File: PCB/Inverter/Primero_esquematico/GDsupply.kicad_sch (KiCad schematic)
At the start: 43 parts, among them T1 750317595, U1 UCC21750QDWRQ1, U2 LM25180QNGURQ1

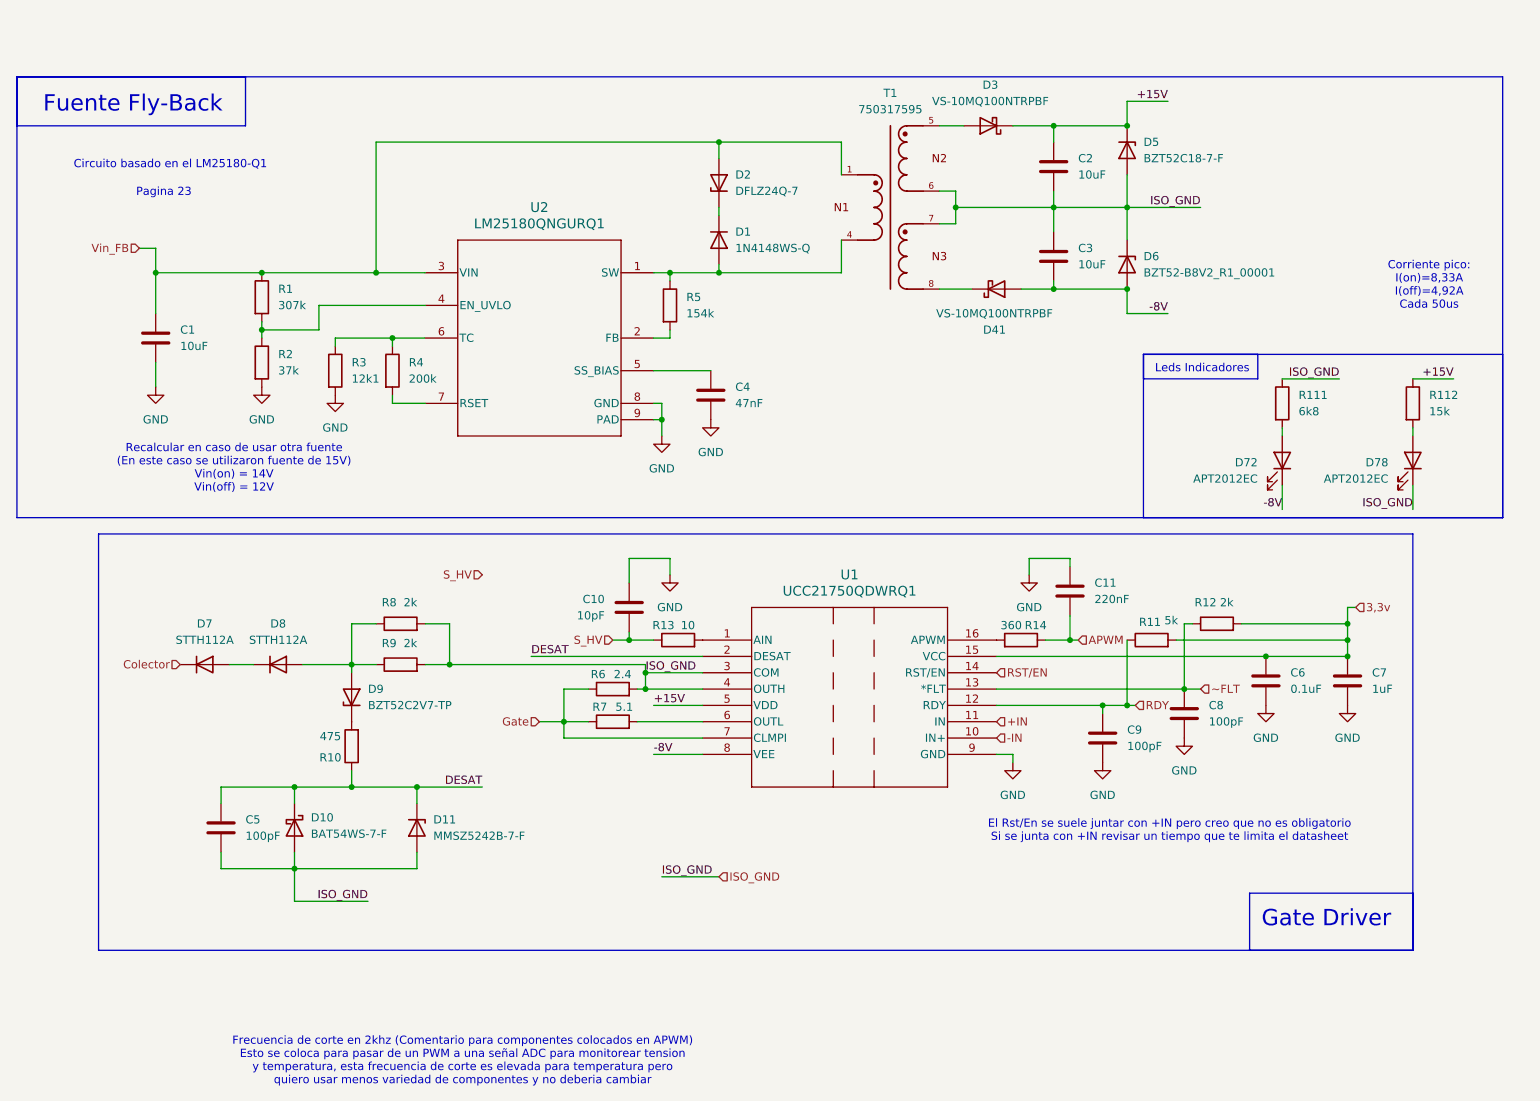
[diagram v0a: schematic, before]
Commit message: Correcciones incompletas e instalaciones de un par de extensiones copadas
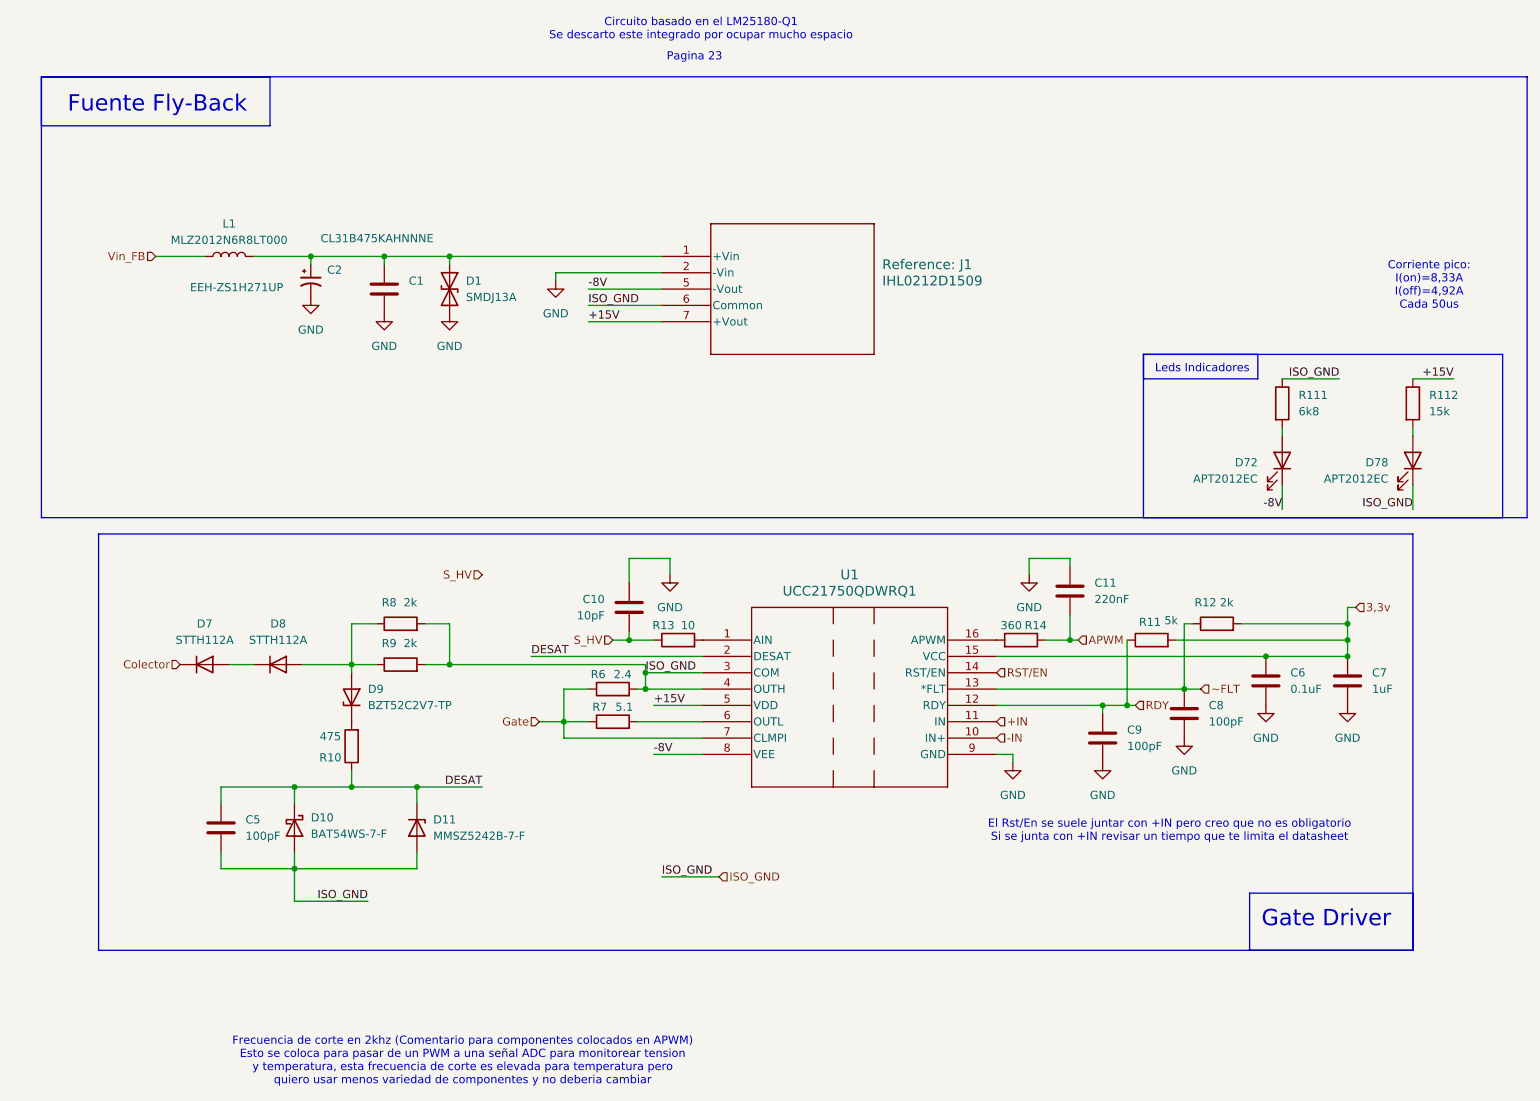
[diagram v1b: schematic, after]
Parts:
- removed C2, C3: 10uF, symbol Device:C
- removed C4: 47nF, symbol Device:C
- removed D1: 1N4148WS-Q, Diode_SMD:D_SOD-323F, symbol Device:D
- removed D2: DFLZ24Q-7, symbol Device:D_Zener
- removed D3, D41: VS-10MQ100NTRPBF, symbol Device:D_Schottky
- removed D5: BZT52C18-7-F, symbol Device:D_Zener
- removed D6: BZT52-B8V2_R1_00001, symbol Device:D_Zener
- removed R1: 307k, symbol Device:R
- removed R2: 37k, symbol Device:R
- removed R3: 12k1, symbol Device:R
- removed R4: 200k, symbol Device:R
- removed R5: 154k, symbol Device:R
- removed T1: 750317595, FSAE-footprints:WE-FLYTI_EP7_4436, symbol Fsae:750317595
- removed U2: LM25180QNGURQ1, NGU0008C, symbol Fsae:LM25180QNGURQ1
- added C2: EEH-ZS1H271UP, Capacitor_SMD:CP_Elec_10x10, symbol Device:C_Polarized_Small_US
- added D1: SMDJ13A, Diode_SMD:D_SMC, symbol Device:D_TVS
- added J1: IHL0212D1509, Snapeda:CONN5_05D1509_XPR, symbol Snapeda:IHL0205D1509
- added L1: MLZ2012N6R8LT000, Inductor_SMD:L_0805_2012Metric, symbol Device:L
- C1: value 10uF -> CL31B475KAHNNNE; footprint (none) -> Capacitor_SMD:C_1206_3216Metric; Compra (none) -> https://www.digikey.com/en/products/detail/samsung-electro-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
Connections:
- net +15V: now also J1.7 (+Vout)
- net -8V: now also J1.5 (-Vout)
- net GND: now also C1.2, C2.2, D1.2 (A2), J1.2 (-Vin); no longer C1.1
- net ISO_GND: now also J1.6 (Common)
- net Vin_FB: now also L1.1; no longer C1.2
- new net: C1.1, C2.1, D1.1 (A1), J1.1 (+Vin), L1.2
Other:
- note added: "Circuito basado en el LM25180-Q1 Se descarto este integrado por ocupar mucho espacio"
- note removed: "Circuito basado en el LM25180-Q1"
- note removed: "Recalcular en caso de usar otra fuente (En este caso se utilizaron fuente de 15V) Vin(on) = 14V Vin(off) = 12V"
